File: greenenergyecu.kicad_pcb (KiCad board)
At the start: 2 copper layers, 34.5 x 35.2 mm, 4 parts, among them M1 Module-vr-discrete-0.5, M2 Module-knock-0.2, M3 Module-vr-0.1, M4 Module-motor-driver-0.1

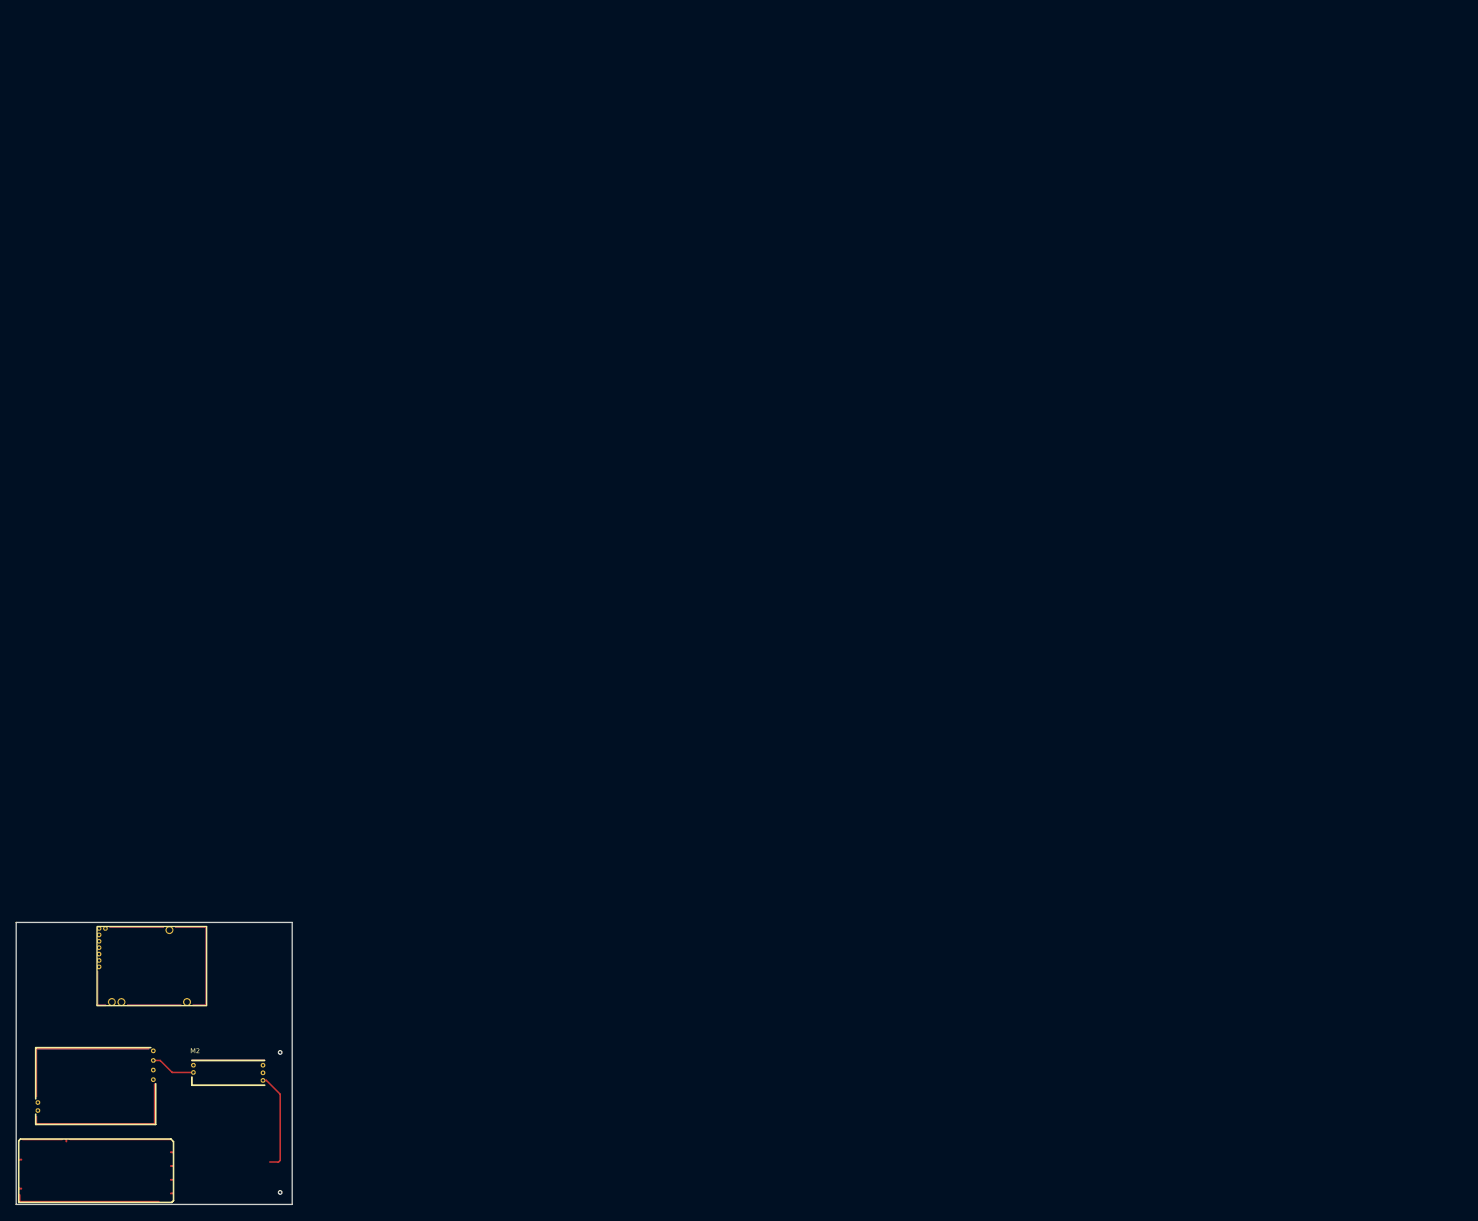
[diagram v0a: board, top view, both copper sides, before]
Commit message: ew
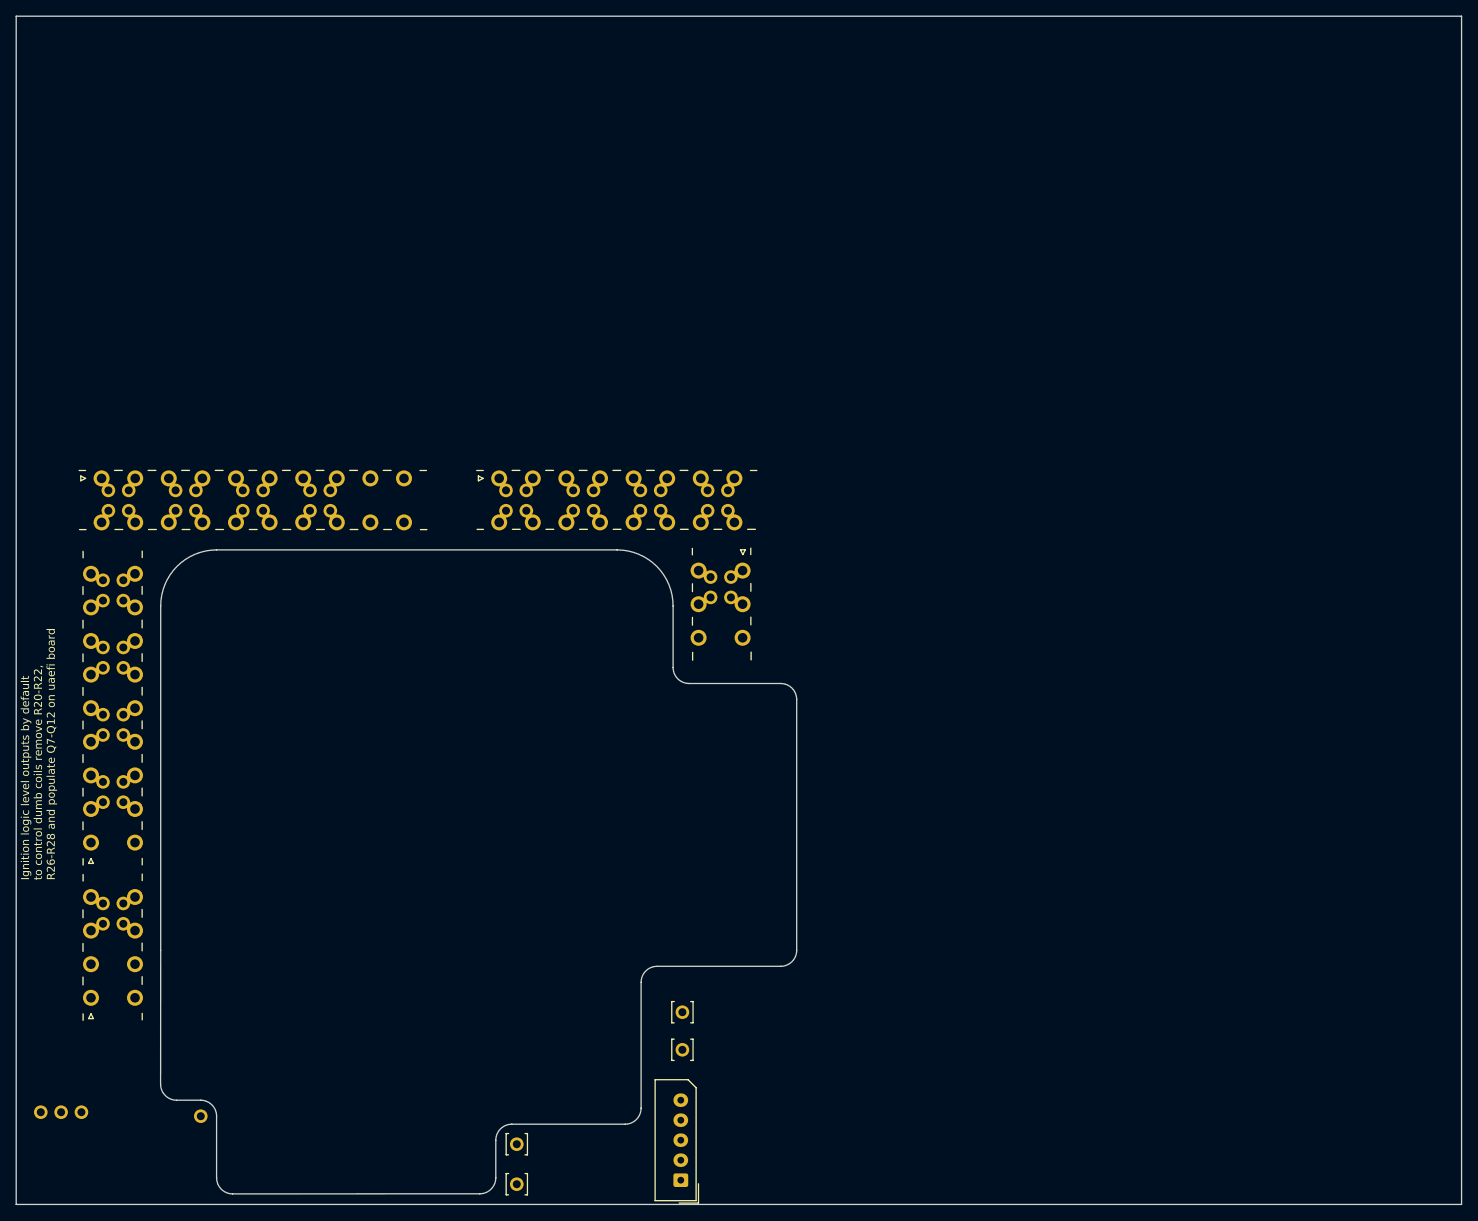
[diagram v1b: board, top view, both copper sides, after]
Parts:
- removed M1: Module-vr-discrete-0.5, hellen-one-vr-discrete-0.5:vr-discrete
- removed M2: Module-knock-0.2, hellen-one-knock-0.2:knock
- removed M3: Module-vr-0.1, hellen-one-vr-0.1:vr
- removed M4: Module-motor-driver-0.1, motor-driver:motor-driver
- added M5: Module:uaefi/0.2, 0.2:uaefi, F.Cu at (0.05, 20.5)
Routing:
- net Net-(M2-OUT_KNOCK): track 12.5 -> 0.00 mm
- net Net-(M1-OUT): track 5.63 -> 0.00 mm
- net (no net): vias 2 -> 0
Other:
- board size 34.5 x 35.2 mm -> 180.7 x 148.5 mm
